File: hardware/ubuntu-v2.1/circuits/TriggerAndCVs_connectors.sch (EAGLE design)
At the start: 11 parts

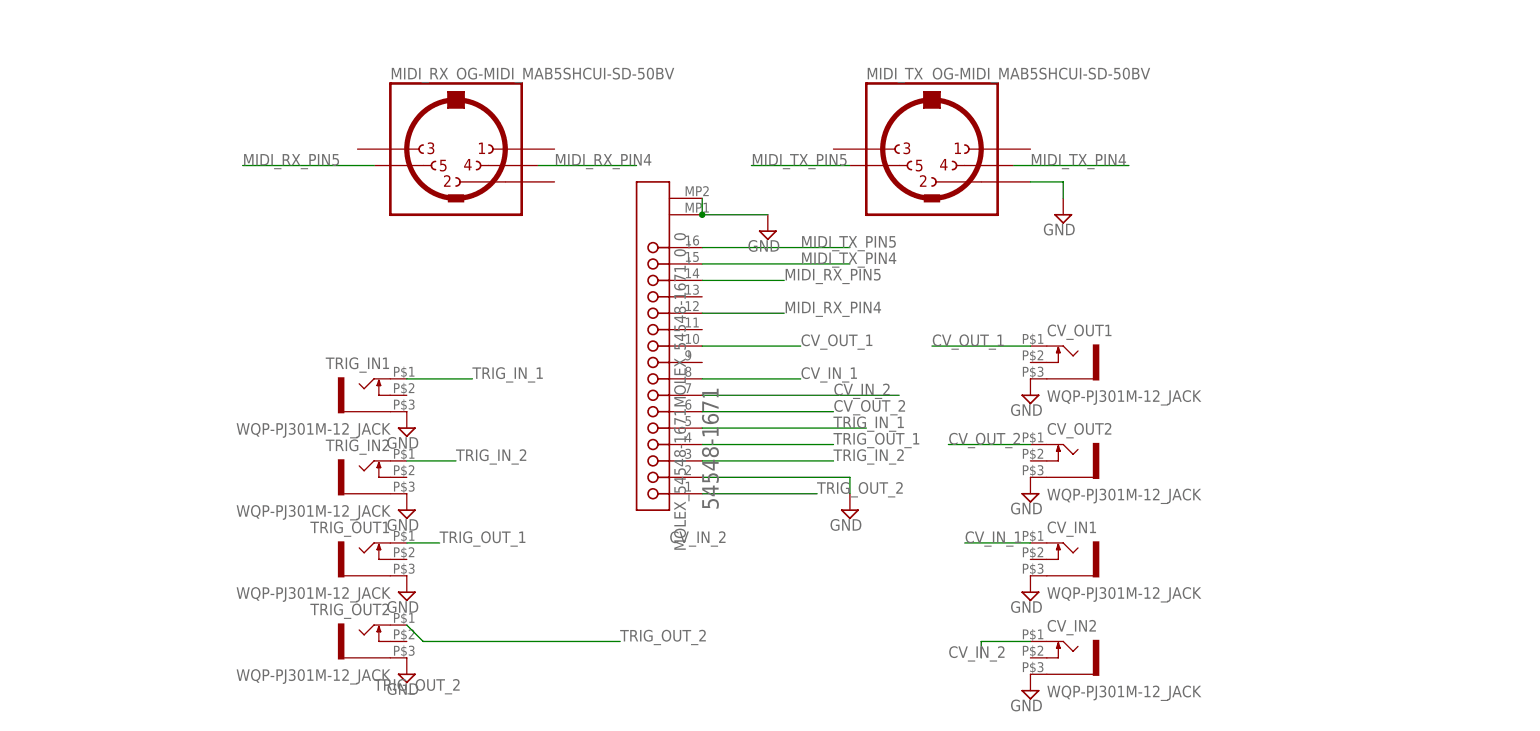
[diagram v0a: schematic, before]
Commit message: Add files via upload
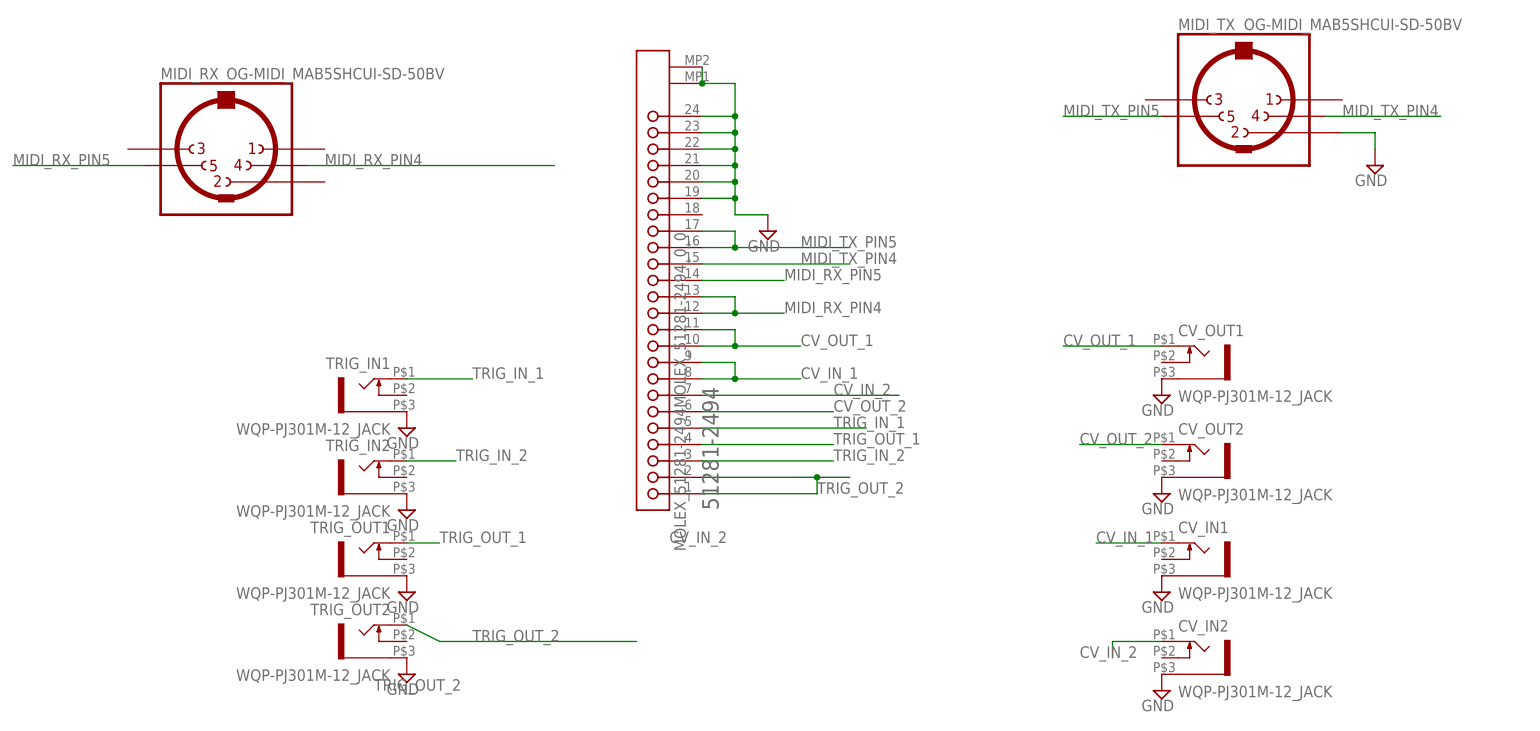
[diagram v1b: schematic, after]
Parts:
- JP4: value MOLEX_54548-1671MOLEX_54548-1671_0_0 -> MOLEX_51281-2494MOLEX_51281-2494_0_0; device Molex - 54548-1671:MOLEX_54548-1671MOLEX_54548-1671_0_0 -> Molex - 51281-2494:MOLEX_51281-2494MOLEX_51281-2494_0_0
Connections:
- net CV_IN_1: now also JP4.9
- net CV_OUT_1: now also JP4.11
- net GND: now also JP4.19, JP4.20, JP4.21, JP4.22, JP4.23, JP4.24; no longer JP4.2
- net MIDI_RX_PIN4: now also JP4.13
- net MIDI_TX_PIN5: now also JP4.17
- net TRIG_OUT_2: now also JP4.2
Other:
- moved on the sheet: CV_IN1, CV_IN2, CV_OUT1, CV_OUT2, MIDI_RX, MIDI_TX
